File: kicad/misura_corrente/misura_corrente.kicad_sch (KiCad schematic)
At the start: 27 parts, among them U0 CA3140, U1 CA3140, U2 INA111, U3 L7808

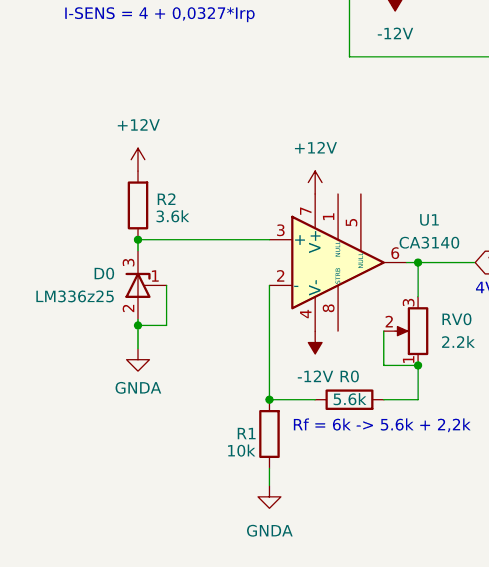
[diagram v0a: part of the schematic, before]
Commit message: configurazione vscode e documento
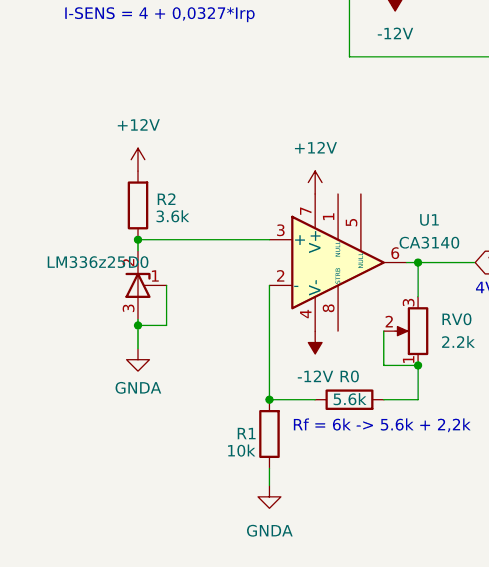
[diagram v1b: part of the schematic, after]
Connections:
- net GNDA: now also D0.3 (V-); no longer D0.2 (V+)
- net at R2.1, U1.3 (+): now also D0.2 (V+); no longer D0.3 (V-)
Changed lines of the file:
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@@
   (symbol (lib_id "simboli_tesina:LM336") (at 26.035 73.66 270) (unit 1)
     (in_bom yes) (on_board yes) (fields_autoplaced)
-    (property "Reference" "D0" (id 0) (at 23.495 72.3899 90)
+    (property "Reference" "D0" (id 0) (at 27.3051 71.12 90)
       (effects (font (size 1.27 1.27)) (justify right))
     )
-    (property "Value" "LM336z25" (id 1) (at 23.495 74.9299 90)
+    (property "Value" "LM336z25" (id 1) (at 24.7651 71.12 90)
       (effects (font (size 1.27 1.27)) (justify right))
     )
-    (property "Footprint" "Package_TO_SOT_THT:TO-92L_Inline" (id 2) (at 31.115 81.28 0)
+    (property "Footprint" "Package_TO_SOT_THT:TO-92L_Inline" (id 2) (at 18.415 78.74 0)
       (effects (font (size 1.27 1.27)) hide)
     )
-    (property "Datasheet" "" (id 3) (at 31.115 81.28 0)
+    (property "Datasheet" "" (id 3) (at 18.415 78.74 0)
       (effects (font (size 1.27 1.27)) hide)
     )
